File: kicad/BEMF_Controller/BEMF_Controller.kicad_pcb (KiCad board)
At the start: 2 copper layers, 164 parts, among them J1 HEADER4VALULOK, J2 HEADER6, J3 FUSE, J4 Coil_A, J5 Coil_B, J6 Coil_C, J7 Vin, Q1 C3M0280090D, Q2 C3M0280090D, Q3 C3M0280090D, Q4 C3M0280090D, Q5 C3M0280090D, Q6 C3M0280090D, U1 RASPBERRY_PICO-NO_DEBUG, U2 INA181, U3 TC1240A, U4 V_REG_78XX, U5 DGD2304, U6 DGD2304, U7 DGD2304

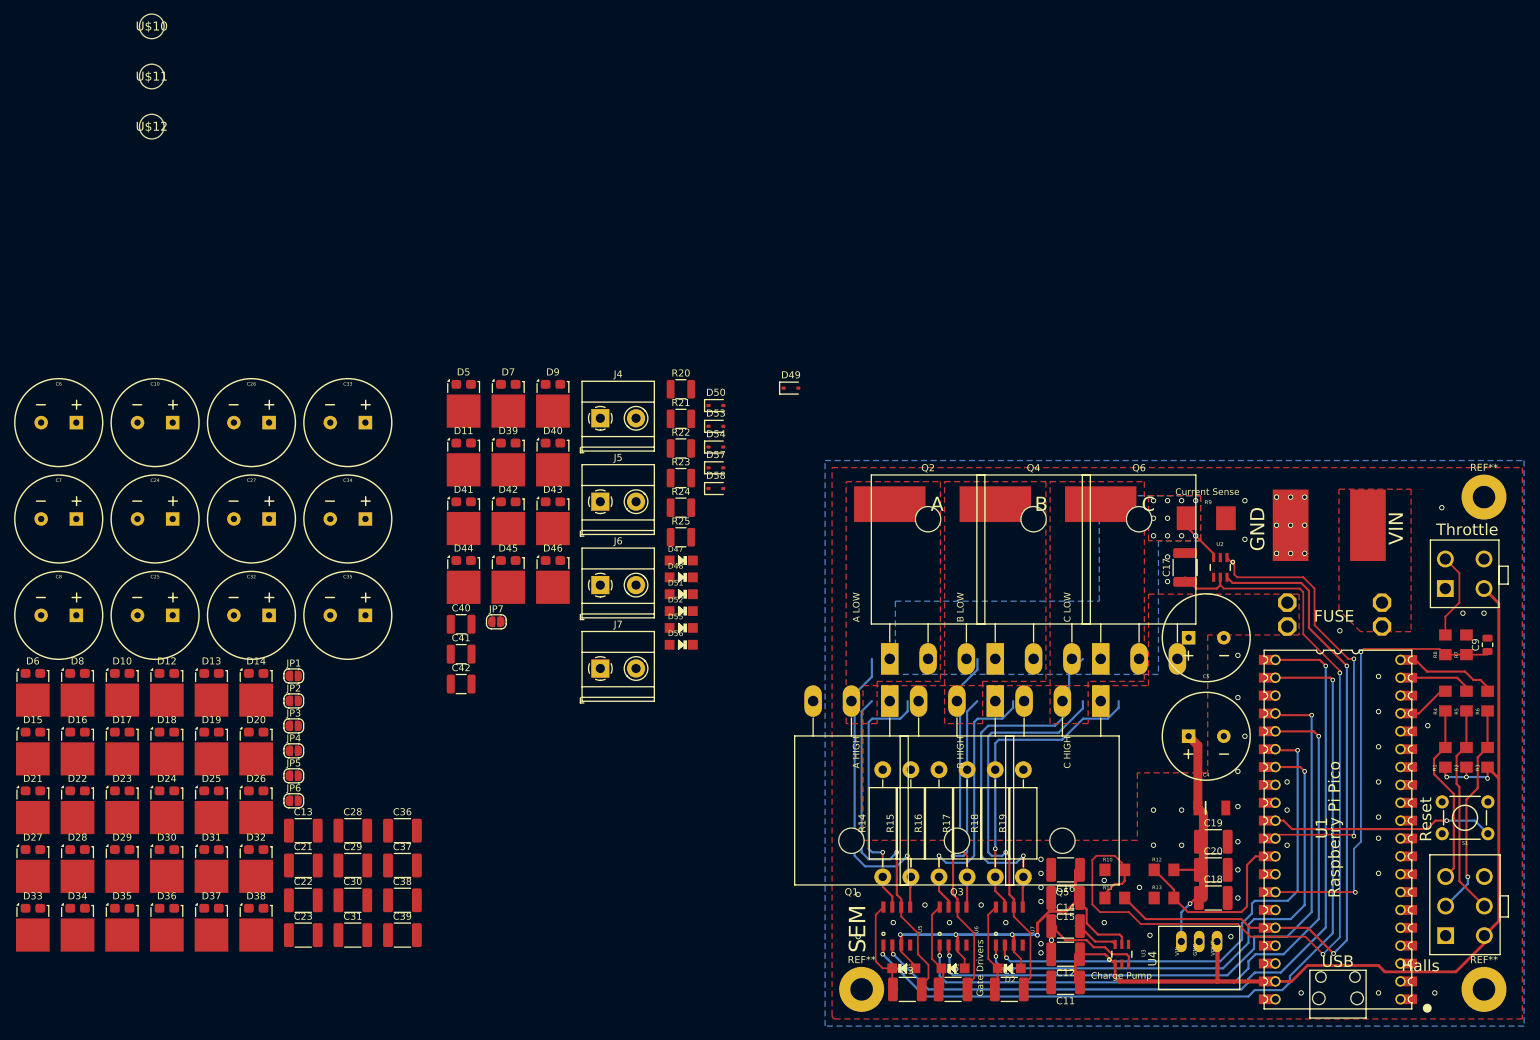
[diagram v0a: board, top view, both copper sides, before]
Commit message: reverted pcb back to original
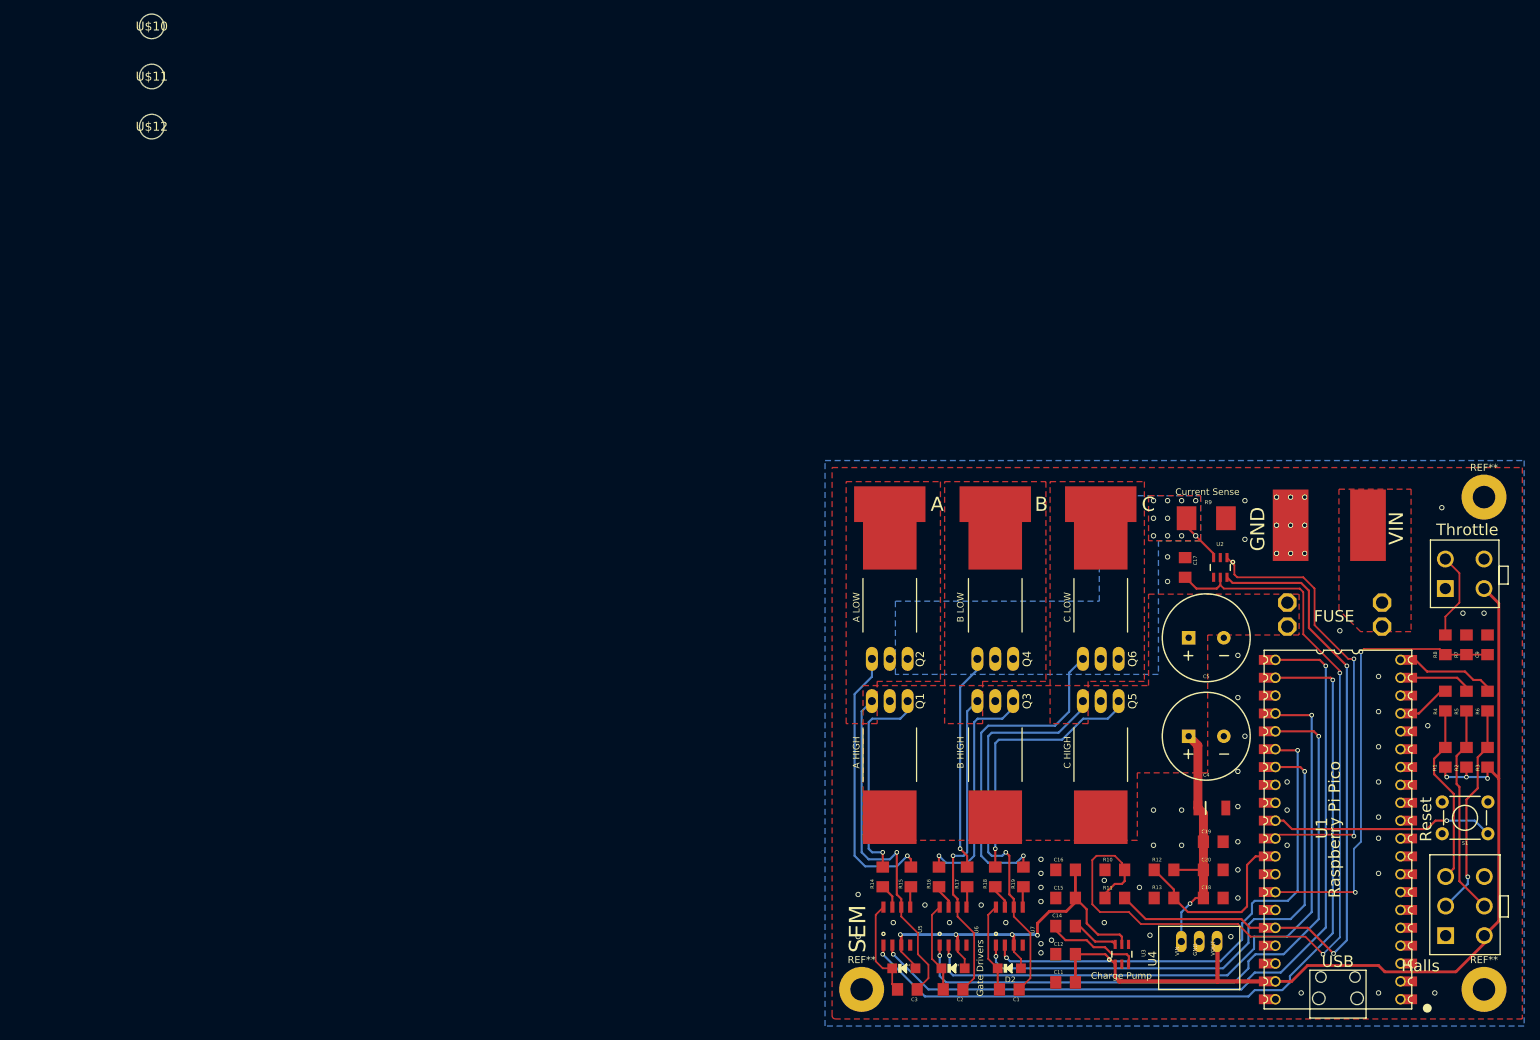
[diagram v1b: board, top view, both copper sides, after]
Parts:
- removed C10, C24, C25, C26, C27, C32, C33, C34, C35, C6, C7, C8: 470uF, main:CPOL-RADIAL-5MM-10MM
- removed C13, C21, C22, C23, C28, C29, C30, C31, C36, C37, C38, C39: 1uF, Capacitor_SMD:C_1812_4532Metric
- removed C40, C41, C42: 1nF/50V, Capacitor_SMD:C_1210_3225Metric
- removed D10, D11, D12, D13, D14, D15, D16, D17, D18, D19, D20, D21, D22, D23, D24, D25, D26, D27, D28, D29, D30, D31, D32, D33, D34, D35, D36, D37, D38, D39, D40, D41, D42, D43, D44, D45, D46, D5, D6, D7, D8, D9: FSV20150V, Package_TO_SOT_SMD:TO-277A
- removed D47, D48, D51, D52, D55, D56: BZT52-B75J, main:SOD-123
- removed D49, D50, D53, D54, D57, D58: 1N4148WS, Diode_SMD:D_SOD-323
- removed J4: Coil_A, TerminalBlock_Phoenix:TerminalBlock_Phoenix_MKDS-1,5-2-5.08_1x02_P5.08mm_Horizontal
- removed J5: Coil_B, TerminalBlock_Phoenix:TerminalBlock_Phoenix_MKDS-1,5-2-5.08_1x02_P5.08mm_Horizontal
- removed J6: Coil_C, TerminalBlock_Phoenix:TerminalBlock_Phoenix_MKDS-1,5-2-5.08_1x02_P5.08mm_Horizontal
- removed J7: Vin, TerminalBlock_Phoenix:TerminalBlock_Phoenix_MKDS-1,5-2-5.08_1x02_P5.08mm_Horizontal
- removed JP1, JP2, JP3, JP4, JP5, JP6, JP7: Jumper, Jumper:SolderJumper-2_P1.3mm_Open_RoundedPad1.0x1.5mm
- removed R20, R21, R22, R23, R24, R25: 10k, Resistor_SMD:R_1210_3225Metric
- C1, C11, C12, C14, C15, C16, C17, C18, C19, C2, C20, C3: footprint Capacitor_SMD:C_1812_4532Metric -> main:1206
- C9: footprint Capacitor_SMD:C_0805_2012Metric -> main:1206
- Q1, Q2, Q3, Q4, Q5, Q6: value C3M0280090D -> MOSFET-NCHANNELTO-220-FLAT; footprint Package_TO_SOT_THT:TO-247-3_Horizontal_TabDown -> main:TO-220-FLAT
- R14, R15, R16, R17, R18, R19: value 10 -> 22; footprint Resistor_THT:R_Axial_DIN0411_L9.9mm_D3.6mm_P15.24mm_Horizontal -> main:1206
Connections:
- net /OVP_A renamed Net-(U1-GP0-Pad1)
- net /OVP_B renamed Net-(U1-GP1-Pad2)
- net /OVP_C renamed Net-(U1-GP2-Pad4)
- C9 pad 1: Net-(C9-Pad1) -> /THROTTLE
- Q1 pad 2: Net-(D9-K) -> /V_RAW
- Q1 pad 3: /SHUNT+ -> /COM_A
- Q2 pad 2: /CAP_BANK_A -> /COM_A
- Q2 pad 3: /COM_A -> /SHUNT+
- Q3 pad 2: /CAP_BANK_B -> /V_RAW
- Q4 pad 2: Net-(D41-K) -> /COM_B
- Q5 pad 2: /CAP_BANK_C -> /V_RAW
- Q6 pad 2: Net-(D45-K) -> /COM_C
- R14 pad 1: Net-(Q2-G) -> /DRV_AH
- R14 pad 2: /DRV_AH -> Net-(Q1-G)
- R15 pad 1: Net-(Q1-G) -> /DRV_AL
- R15 pad 2: /DRV_AL -> Net-(Q2-G)
- R16 pad 1: Net-(Q3-G) -> /DRV_BH
- R16 pad 2: /DRV_BH -> Net-(Q3-G)
- R17 pad 1: Net-(Q4-G) -> /DRV_BL
- R17 pad 2: /DRV_BL -> Net-(Q4-G)
- R18 pad 1: Net-(Q5-G) -> /DRV_CH
- R18 pad 2: /DRV_CH -> Net-(Q5-G)
- R19 pad 1: Net-(Q6-G) -> /DRV_CL
- R19 pad 2: /DRV_CL -> Net-(Q6-G)
- R8 pad 2: Net-(C9-Pad1) -> /THROTTLE
- U4 pad IN: Net-(J7-Pin_1) -> /V_RAW
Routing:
- net Net-(Q2-G): track 0.00 -> 39.6 mm, vias 0 -> 1
- net Net-(D9-K): track 39.6 -> 0.00 mm, vias 1 -> 0
